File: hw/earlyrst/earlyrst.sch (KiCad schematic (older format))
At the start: 5 parts, among them U1 74LS04, U2 74LS32, U3 74LS193, U4 74LS541, U5 74LS175

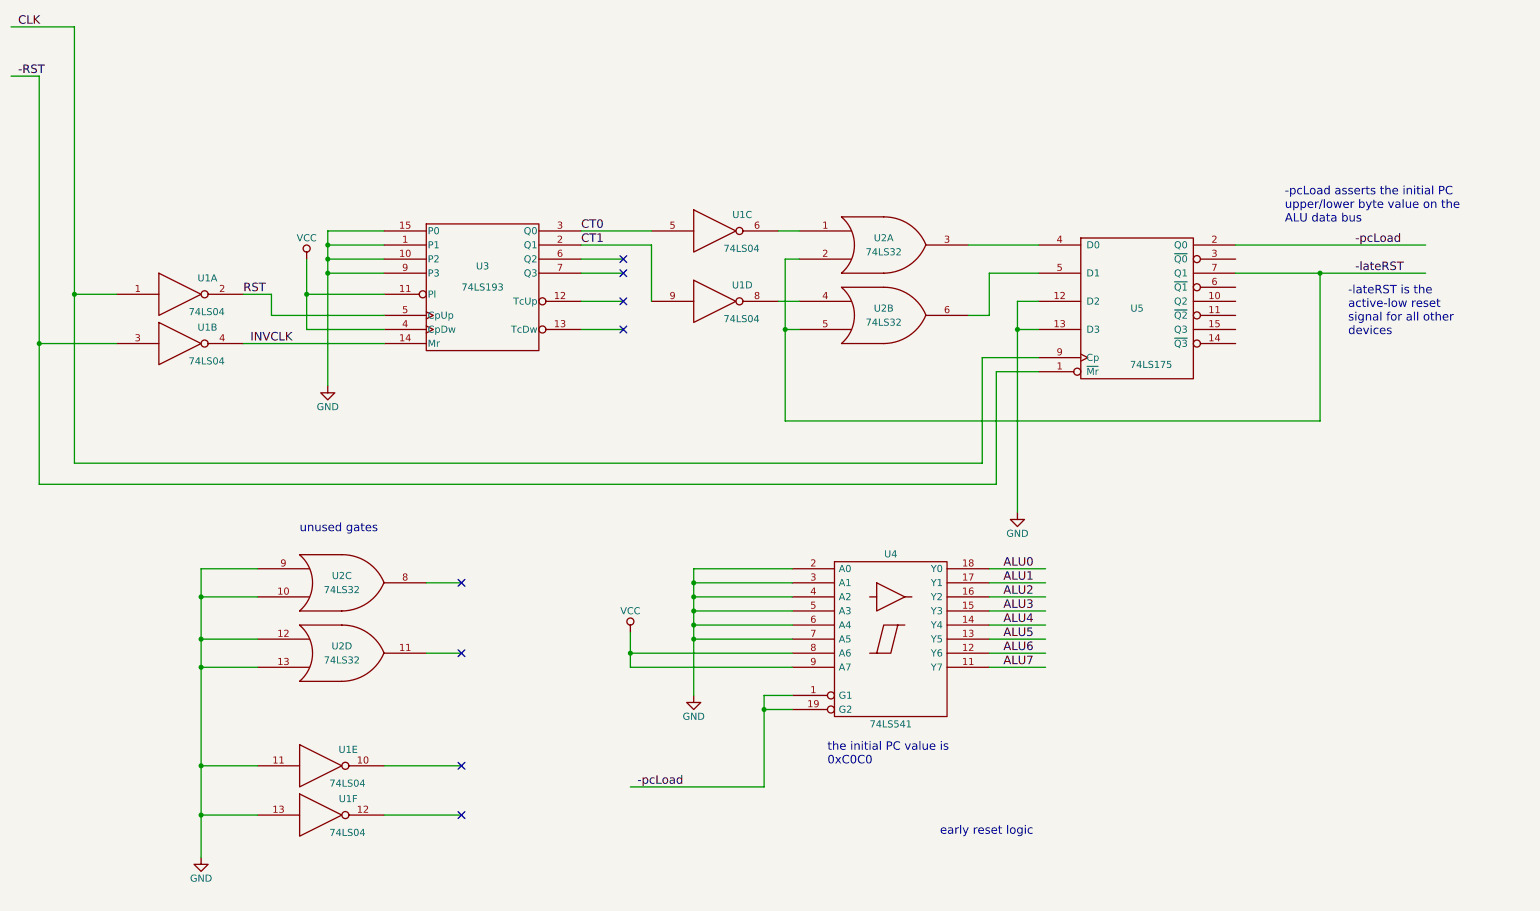
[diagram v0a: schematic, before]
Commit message: finally, a working version
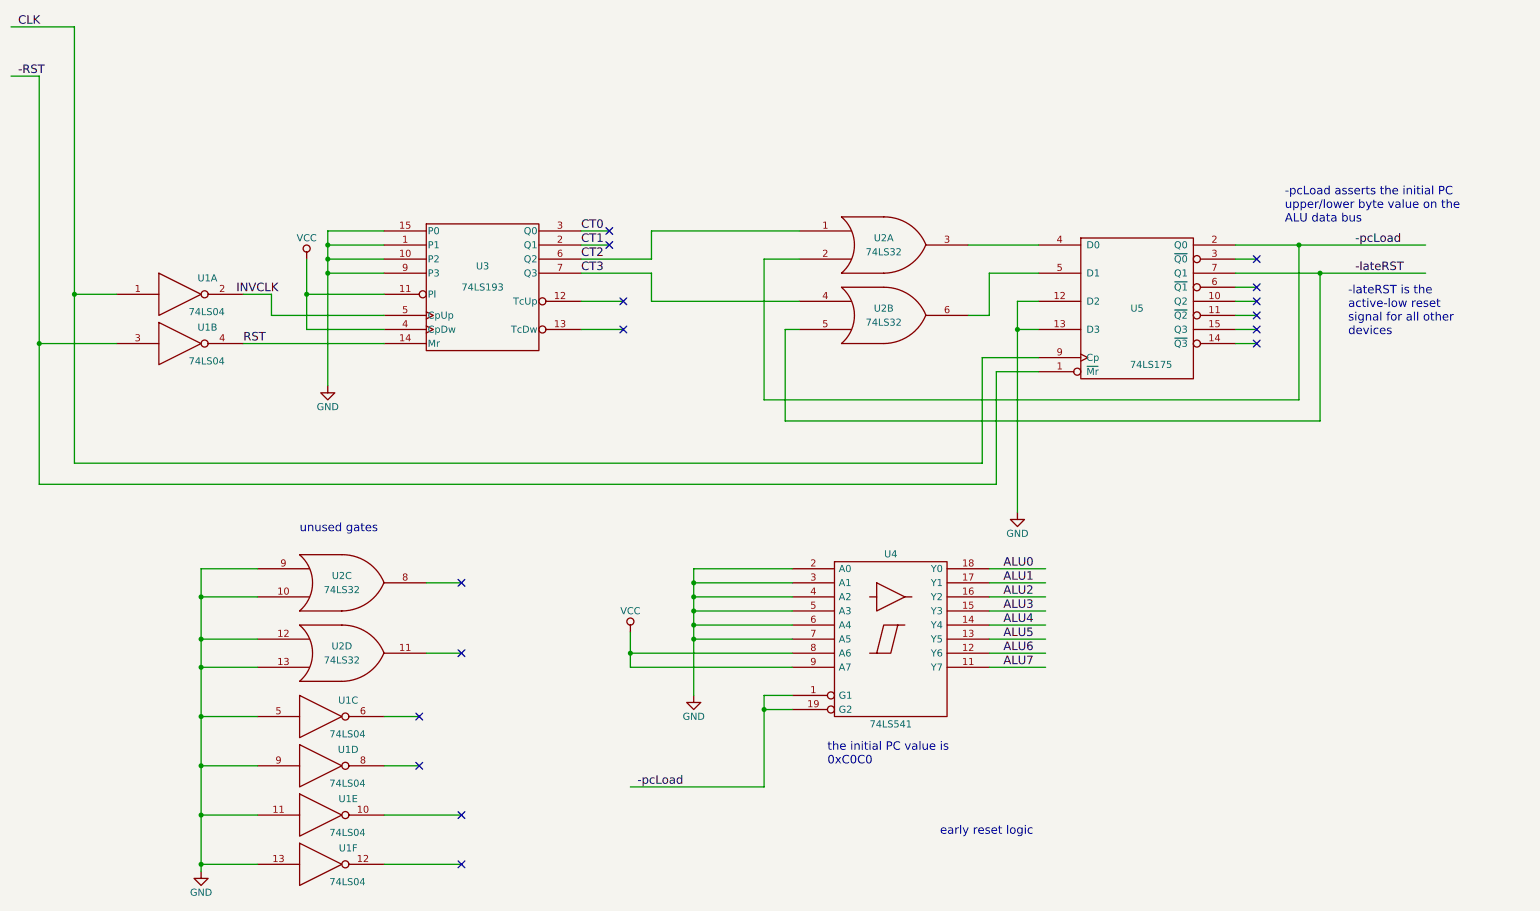
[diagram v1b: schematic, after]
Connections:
- net labels added: CT2, CT3
- wire segments 80 -> 94
- no-connect marks 8 -> 16
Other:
- moved on the sheet: U1C, U1D, U1E, U1F
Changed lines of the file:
@@
 NoConn ~ 4900 3000
 NoConn ~ 4900 3200
-NoConn ~ 4900 2700
-NoConn ~ 4900 2800
 $Comp
 L 74LS32 U2
@@
 L 74LS04 U1
 U 5 1 59259341
-P 2750 6300
-F 0 "U1" H 2945 6415 50  0000 C CNN
-F 1 "74LS04" H 2940 6175 50  0000 C CNN
-F 2 "" H 2750 6300 50  0001 C CNN
-F 3 "" H 2750 6300 50  0001 C CNN
-	5    2750 6300
+P 2750 6650
+F 0 "U1" H 2945 6765 50  0000 C CNN
+F 1 "74LS04" H 2940 6525 50  0000 C CNN
+F 2 "" H 2750 6650 50  0001 C CNN
+F 3 "" H 2750 6650 50  0001 C CNN
+	5    2750 6650
 	1    0    0    -1
 $EndComp
@@
 Text Label 600  1400 0    60   ~ 0
 -RST
-Text Label 2200 2950 0    60   ~ 0
-RST
-Text Label 2250 3300 0    60   ~ 0
-INVCLK
 $Comp
 L 74LS32 U2
@@
 L 74LS04 U1
 U 6 1 5925A468
-P 2750 6650
-F 0 "U1" H 2945 6765 50  0000 C CNN
-F 1 "74LS04" H 2940 6525 50  0000 C CNN
-F 2 "" H 2750 6650 50  0001 C CNN
-F 3 "" H 2750 6650 50  0001 C CNN
-	6    2750 6650
+P 2750 7000
+F 0 "U1" H 2945 7115 50  0000 C CNN
+F 1 "74LS04" H 2940 6875 50  0000 C CNN
+F 2 "" H 2750 7000 50  0001 C CNN
+F 3 "" H 2750 7000 50  0001 C CNN
+	6    2750 7000
 	1    0    0    -1
 $EndComp
@@
 L 74LS04 U1
 U 3 1 5925A4A5
-P 5550 2500
-F 0 "U1" H 5745 2615 50  0000 C CNN
-F 1 "74LS04" H 5740 2375 50  0000 C CNN
-F 2 "" H 5550 2500 50  0001 C CNN
-F 3 "" H 5550 2500 50  0001 C CNN
-	3    5550 2500
+P 2750 5950
+F 0 "U1" H 2945 6065 50  0000 C CNN
+F 1 "74LS04" H 2940 5825 50  0000 C CNN
+F 2 "" H 2750 5950 50  0001 C CNN
+F 3 "" H 2750 5950 50  0001 C CNN
+	3    2750 5950
 	1    0    0    -1
 $EndComp
@@
 L 74LS04 U1
 U 4 1 5925A4D4
-P 5550 3000
-F 0 "U1" H 5745 3115 50  0000 C CNN
-F 1 "74LS04" H 5740 2875 50  0000 C CNN
-F 2 "" H 5550 3000 50  0001 C CNN
-F 3 "" H 5550 3000 50  0001 C CNN
-	4    5550 3000
+P 2750 6300
+F 0 "U1" H 2945 6415 50  0000 C CNN
+F 1 "74LS04" H 2940 6175 50  0000 C CNN
+F 2 "" H 2750 6300 50  0001 C CNN
+F 3 "" H 2750 6300 50  0001 C CNN
+	4    2750 6300
 	1    0    0    -1
 $EndComp
@@
 L GND #PWR1
 U 1 1 5925AADF
-P 1900 6950
-F 0 "#PWR1" H 1900 6700 50  0001 C CNN
-F 1 "GND" H 1900 6800 50  0000 C CNN
-F 2 "" H 1900 6950 50  0001 C CNN
-F 3 "" H 1900 6950 50  0001 C CNN
-	1    1900 6950
+P 1900 7050
+F 0 "#PWR1" H 1900 6800 50  0001 C CNN
+F 1 "GND" H 1900 6900 50  0000 C CNN
+F 2 "" H 1900 7050 50  0001 C CNN
+F 3 "" H 1900 7050 50  0001 C CNN
+	1    1900 7050
 	1    0    0    -1
 $EndComp
 NoConn ~ 3750 5500
-NoConn ~ 3750 6300
 NoConn ~ 3750 6650
+NoConn ~ 3750 7000
 Text Notes 2600 4650 0    60   ~ 0
 unused gates
@@
 	4600 3200 4900 3200
 Wire Wire Line
-	4600 2800 4900 2800
-Wire Wire Line
-	4600 2700 4900 2700
-Wire Wire Line
 	7350 2600 7850 2600
 Wire Wire Line
@@
 	2300 5400 1900 5400
 Wire Wire Line
-	1900 4900 1900 6950
+	1900 4900 1900 7050
 Wire Wire Line
 	2300 5600 1900 5600
 Connection ~ 1900 5600
 Wire Wire Line
-	2300 6300 1900 6300
-Connection ~ 1900 6300
-Wire Wire Line
 	2300 6650 1900 6650
-Connection ~ 1900 6650
+Wire Wire Line
+	2300 7000 1900 7000
 Wire Wire Line
 	3500 5500 3750 5500
 Wire Wire Line
-	3200 6300 3750 6300
-Wire Wire Line
 	3200 6650 3750 6650
+Wire Wire Line
+	3200 7000 3750 7000
 Wire Wire Line
 	6100 5600 4950 5600
@@
 -pcLoad
 Wire Wire Line
-	6150 2500 6000 2500
+	5100 2500 6150 2500
 Wire Wire Line
 	7850 3000 7700 3000
@@
 Connection ~ 7700 3200
 Wire Wire Line
-	4600 2500 5100 2500
-Wire Wire Line
-	4600 2600 5100 2600
-Wire Wire Line
-	5100 2600 5100 3000
-Text Label 4600 2500 0    60   ~ 0
-CT0
-Text Label 4600 2600 0    60   ~ 0
-CT1
-Wire Wire Line
-	6000 3000 6150 3000
+	5100 3000 6150 3000
 Wire Wire Line
 	7850 3500 7550 3500
@@
 	9850 3850 6050 3850
 Wire Wire Line
-	6050 3850 6050 2700
-Wire Wire Line
-	6050 2700 6150 2700
+	5900 2700 6150 2700
 Wire Wire Line
 	6150 3200 6050 3200
-Connection ~ 6050 3200
 Wire Wire Line
 	7350 3100 7500 3100
@@
 Wire Wire Line
 	3500 5000 3750 5000
+NoConn ~ 3450 5950
+Wire Wire Line
+	3200 5950 3450 5950
+NoConn ~ 3450 6300
+Wire Wire Line
+	3200 6300 3450 6300
+Wire Wire Line
+	2300 5950 1900 5950
+Connection ~ 1900 5950
+Wire Wire Line
+	2300 6300 1900 6300
+Connection ~ 1900 6300
+Connection ~ 1900 6650
+Connection ~ 1900 7000
+Wire Wire Line
+	6050 3200 6050 3850
+Wire Wire Line
+	5900 2700 5900 3700
+Wire Wire Line
+	5900 3700 9700 3700
+Wire Wire Line
+	9700 3700 9700 2600
+Connection ~ 9700 2600
+Wire Wire Line
+	4600 2500 4800 2500
+Wire Wire Line
+	4600 2600 4800 2600
+Wire Wire Line
+	4600 2700 5100 2700
+Wire Wire Line
+	4600 2800 5100 2800
+Text Label 4600 2500 0    60   ~ 0
+CT0
+Text Label 4600 2600 0    60   ~ 0
+CT1
+Text Label 4600 2700 0    60   ~ 0
+CT2
+Text Label 4600 2800 0    60   ~ 0
+CT3
+NoConn ~ 4800 2500
+NoConn ~ 4800 2600
+Wire Wire Line
+	5100 2700 5100 2500
+Wire Wire Line
+	5100 2800 5100 3000
+Text Label 2150 2950 0    60   ~ 0
+INVCLK
+Text Label 2200 3300 0    60   ~ 0
+RST
+Wire Wire Line
+	9250 2700 9400 2700
+Wire Wire Line
+	9250 2900 9400 2900
+Wire Wire Line
+	9250 3000 9400 3000
+Wire Wire Line
+	9250 3100 9400 3100
+Wire Wire Line
+	9250 3200 9400 3200
+Wire Wire Line
+	9250 3300 9400 3300
+NoConn ~ 9400 2700
+NoConn ~ 9400 2900
+NoConn ~ 9400 3000
+NoConn ~ 9400 3100
+NoConn ~ 9400 3200
+NoConn ~ 9400 3300
 $EndSCHEMATC
